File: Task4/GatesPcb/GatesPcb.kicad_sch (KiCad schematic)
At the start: 11 parts, among them J1 S2B-PH-K-SLFSN, J2 ON/OFF, U1 ESP32-S2-SOLO, U2 LM317_SOT-223, U3 UART

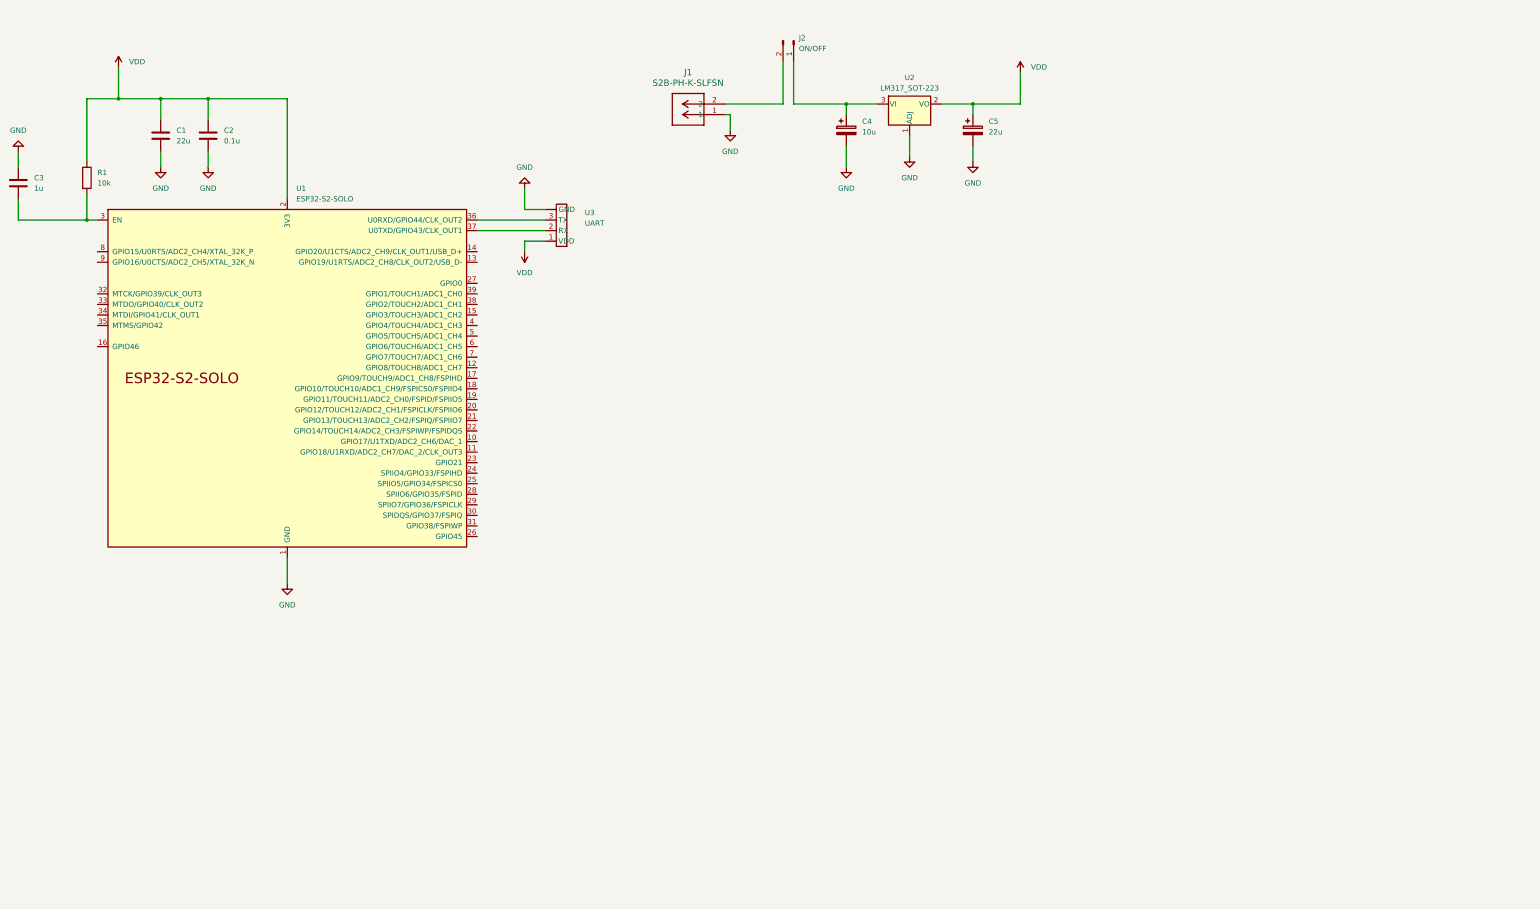
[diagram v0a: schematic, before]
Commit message: finished first pcb hopefully it works ...
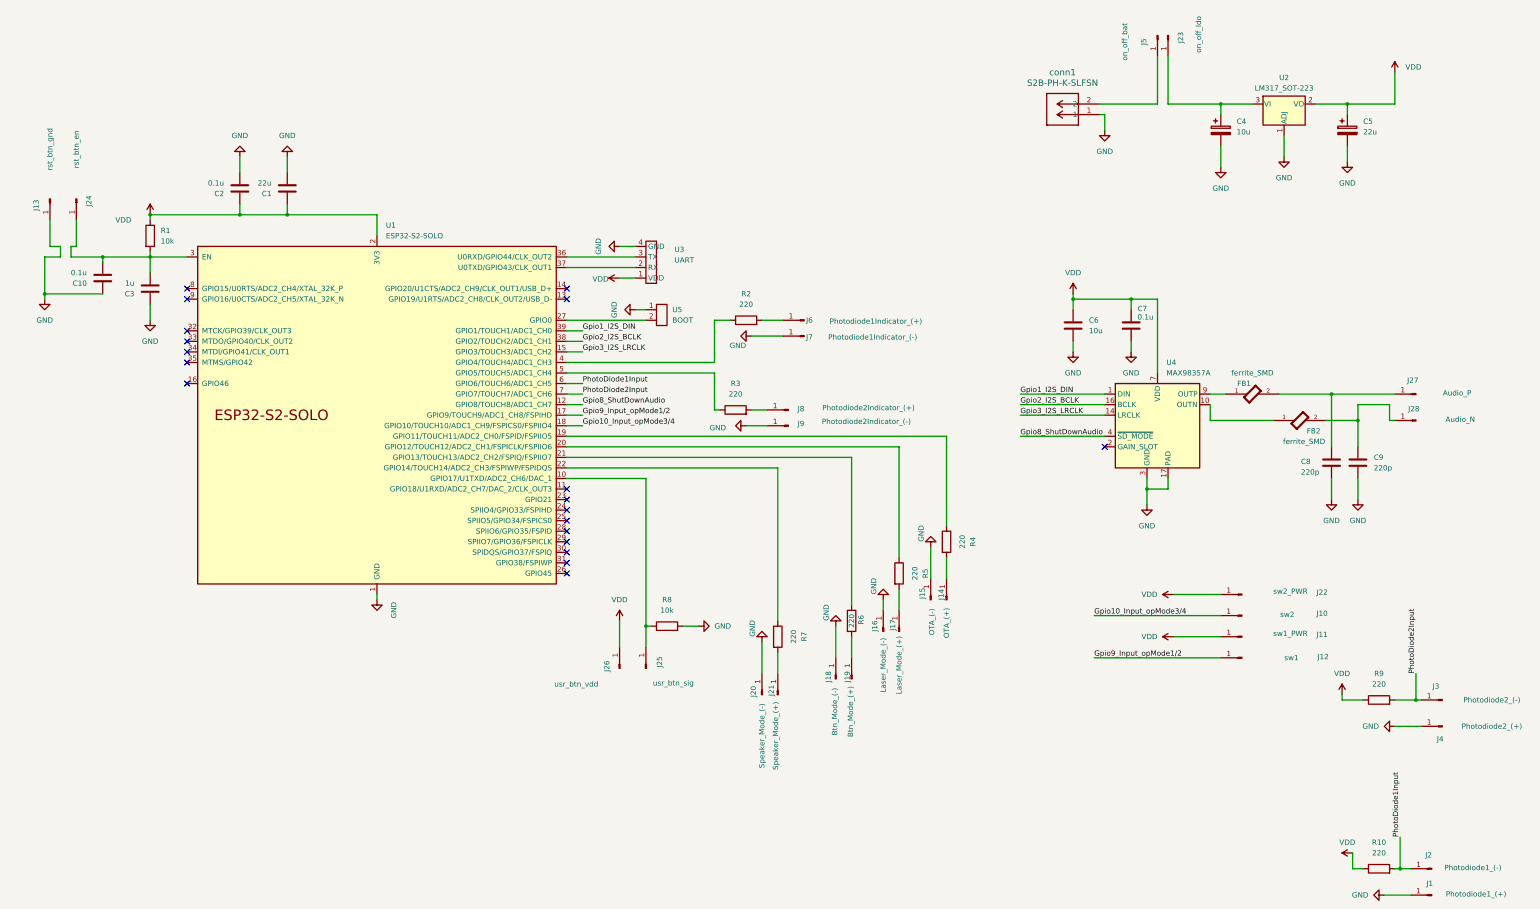
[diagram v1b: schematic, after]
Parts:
- removed J2: ON/OFF, symbol Connector:Conn_01x02_Pin
- added C10, C7: 0.1u, Capacitor_SMD:C_1206_3216Metric, symbol Device:C
- added C6: 10u, Capacitor_SMD:C_1206_3216Metric, symbol Device:C
- added C8, C9: 220p, Capacitor_SMD:C_1206_3216Metric, symbol Device:C
- added FB1, FB2: ferrite_SMD, laserGatesFootprints:FB_HI1206P121R-10, symbol MURATA_BLM18KN471EH1D:MURATA_BLM18KN471EH1D
- added J1: Photodiode1_(+), laserGatesFootprints:+_connectorPad, symbol Connector:Conn_01x01_Pin
- added J10: sw2, laserGatesFootprints:-_connectorPad, symbol Connector:Conn_01x01_Pin
- added J11: sw1_PWR, laserGatesFootprints:+_connectorPad, symbol Connector:Conn_01x01_Pin
- added J12: sw1, laserGatesFootprints:-_connectorPad, symbol Connector:Conn_01x01_Pin
- added J13: rst_btn_gnd, laserGatesFootprints:-_connectorPad, symbol Connector:Conn_01x01_Pin
- added J14: OTA_(+), laserGatesFootprints:+_connectorPad, symbol Connector:Conn_01x01_Pin
- added J15: OTA_(-), laserGatesFootprints:-_connectorPad, symbol Connector:Conn_01x01_Pin
- added J16: Laser_Mode_(-), laserGatesFootprints:-_connectorPad, symbol Connector:Conn_01x01_Pin
- added J17: Laser_Mode_(+), laserGatesFootprints:+_connectorPad, symbol Connector:Conn_01x01_Pin
- added J18: Btn_Mode_(-), laserGatesFootprints:-_connectorPad, symbol Connector:Conn_01x01_Pin
- added J19: Btn_Mode_(+), laserGatesFootprints:+_connectorPad, symbol Connector:Conn_01x01_Pin
- added J2: Photodiode1_(-), laserGatesFootprints:-_connectorPad, symbol Connector:Conn_01x01_Pin
- added J20: Speaker_Mode_(-), laserGatesFootprints:-_connectorPad, symbol Connector:Conn_01x01_Pin
- added J21: Speaker_Mode_(+), laserGatesFootprints:+_connectorPad, symbol Connector:Conn_01x01_Pin
- added J22: sw2_PWR, laserGatesFootprints:+_connectorPad, symbol Connector:Conn_01x01_Pin
- added J23: on_off_ldo, laserGatesFootprints:-_connectorPad, symbol Connector:Conn_01x01_Pin
- added J24: rst_btn_en, laserGatesFootprints:+_connectorPad, symbol Connector:Conn_01x01_Pin
- added J25: usr_btn_sig, laserGatesFootprints:-_connectorPad, symbol Connector:Conn_01x01_Pin
- added J26: usr_btn_vdd, laserGatesFootprints:+_connectorPad, symbol Connector:Conn_01x01_Pin
- added J27: Audio_P, laserGatesFootprints:+_connectorPad, symbol Connector:Conn_01x01_Pin
- added J28: Audio_N, laserGatesFootprints:-_connectorPad, symbol Connector:Conn_01x01_Pin
- added J3: Photodiode2_(-), laserGatesFootprints:-_connectorPad, symbol Connector:Conn_01x01_Pin
- added J4: Photodiode2_(+), laserGatesFootprints:+_connectorPad, symbol Connector:Conn_01x01_Pin
- added J5: on_off_bat, laserGatesFootprints:+_connectorPad, symbol Connector:Conn_01x01_Pin
- added J6: Photodiode1Indicator_(+), laserGatesFootprints:+_connectorPad, symbol Connector:Conn_01x01_Pin
- added J7: Photodiode1Indicator_(-), laserGatesFootprints:-_connectorPad, symbol Connector:Conn_01x01_Pin
- added J8: Photodiode2Indicator_(+), laserGatesFootprints:+_connectorPad, symbol Connector:Conn_01x01_Pin
- added J9: Photodiode2Indicator_(-), laserGatesFootprints:-_connectorPad, symbol Connector:Conn_01x01_Pin
- added R10, R2, R3, R4, R5, R6, R7, R9: 220, Resistor_SMD:R_1206_3216Metric, symbol Device:R
- added R8: 10k, Resistor_SMD:R_1206_3216Metric, symbol Device:R
- added U4: MAX98357A, Package_DFN_QFN:TQFN-16-1EP_3x3mm_P0.5mm_EP1.23x1.23mm, symbol Audio:MAX98357A
- added U5: BOOT, laserGatesFootprints:BOOT_Connectors_Place, symbol connectors:BOOT
- C1, C2, C3: footprint (none) -> Capacitor_SMD:C_1206_3216Metric
- C4, C5: footprint (none) -> laserGatesFootprints:CAPMP3216X180N
- R1: footprint (none) -> Resistor_SMD:R_1206_3216Metric
- U3: footprint (none) -> laserGatesFootprints:UART_Connectors_Place
- conn1: renamed from J1; footprint CONN_S2B-PH-K-S_JST -> laserGatesFootprints:CONN_S2B-PH-K-S_JST
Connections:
- net GND: now also U3.4 (GND), C10.2, C6.1, C7.2, C8.1, C9.1, J1.1 (Pin_1), J13.1 (Pin_1), J15.1 (Pin_1), J16.1 (Pin_1), J18.1 (Pin_1), J20.1 (Pin_1), J4.1 (Pin_1), J7.1 (Pin_1), J9.1 (Pin_1), R8.2, U4.11 (GND), U4.15 (GND), U4.17 (PAD), U4.3 (GND), U5.1; no longer U3. (GND)
- net VDD: now also C6.2, C7.1, J11.1 (Pin_1), J22.1 (Pin_1), J26.1 (Pin_1), R10.1, R9.1, U4.7 (VDD), U4.8 (VDD)
- net at C3.2, R1.2, U1.3 (EN): now also C10.1, J24.1 (Pin_1)
- net at C4.1, U2.3 (VI): now also J23.1 (Pin_1)
- net at conn1.2: now also J5.1 (Pin_1)
- net at U1.10 (GPIO17/U1TXD/ADC2_CH6/DAC_1): now also J25.1 (Pin_1), R8.1
- net Gpio8_ShutDownAudio: now reaches U1.12 (GPIO8/TOUCH8/ADC1_CH7)
- net Gpio8_ShutDownAudio: now also U4.4 (~{SD_MODE})
- net Gpio3_I2S_LRCLK: now reaches U1.15 (GPIO3/TOUCH3/ADC1_CH2)
- net Gpio3_I2S_LRCLK: now also U4.14 (LRCLK)
- net Gpio9_Input_opMode1/2: now reaches U1.17 (GPIO9/TOUCH9/ADC1_CH8/FSPIHD)
- net Gpio9_Input_opMode1/2: now also J12.1 (Pin_1)
- net Gpio10_Input_opMode3/4: now reaches U1.18 (GPIO10/TOUCH10/ADC1_CH9/FSPICS0/FSPIIO4)
- net Gpio10_Input_opMode3/4: now also J10.1 (Pin_1)
- net at U1.19 (GPIO11/TOUCH11/ADC2_CH0/FSPID/FSPIIO5): now also R4.1
- net at U1.20 (GPIO12/TOUCH12/ADC2_CH1/FSPICLK/FSPIIO6): now also R5.1
- net at U1.21 (GPIO13/TOUCH13/ADC2_CH2/FSPIQ/FSPIIO7): now also R6.1
- net at U1.22 (GPIO14/TOUCH14/ADC2_CH3/FSPIWP/FSPIDQS): now also R7.1
- net at U1.27 (GPIO0): now also U5.2
- net Gpio2_I2S_BCLK: now reaches U1.38 (GPIO2/TOUCH2/ADC1_CH1)
- net Gpio2_I2S_BCLK: now also U4.16 (BCLK)
- net Gpio1_I2S_DIN: now reaches U1.39 (GPIO1/TOUCH1/ADC1_CH0)
- net Gpio1_I2S_DIN: now also U4.1 (DIN)
- net at U1.4 (GPIO4/TOUCH4/ADC1_CH3): now also R2.1
- net at U1.5 (GPIO5/TOUCH5/ADC1_CH4): now also R3.1
- net PhotoDiode1Input: now reaches U1.6 (GPIO6/TOUCH6/ADC1_CH5)
- net PhotoDiode1Input: now also J2.1 (Pin_1), R10.2
- net PhotoDiode2Input: now reaches U1.7 (GPIO7/TOUCH7/ADC1_CH6)
- net PhotoDiode2Input: now also J3.1 (Pin_1), R9.2
- new net: J17.1 (Pin_1), R5.2
- new net: J14.1 (Pin_1), R4.2
- new net: C8.2, FB1.2, J27.1 (Pin_1)
- new net: C9.2, FB2.2, J28.1 (Pin_1)
- new net: J21.1 (Pin_1), R7.2
- new net: FB1.1, U4.9 (OUTP)
- new net: J8.1 (Pin_1), R3.2
- new net: FB2.1, U4.10 (OUTN)
- new net: J19.1 (Pin_1), R6.2
- new net: J6.1 (Pin_1), R2.2
- no-connect marks 0 -> 19
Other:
- title: (none) -> Sprinting Gates schematics
- moved on the sheet: C1, C2, C3, C4, C5, R1, U1, U2, conn1
